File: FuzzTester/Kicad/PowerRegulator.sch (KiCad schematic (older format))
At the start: 18 parts, among them J5 TestPower_PinHeader, J6 9V Power JST XH, U1 AMS1117-5.0, U2 AMS1117-3.3, U22 LM2576HVS-ADJ

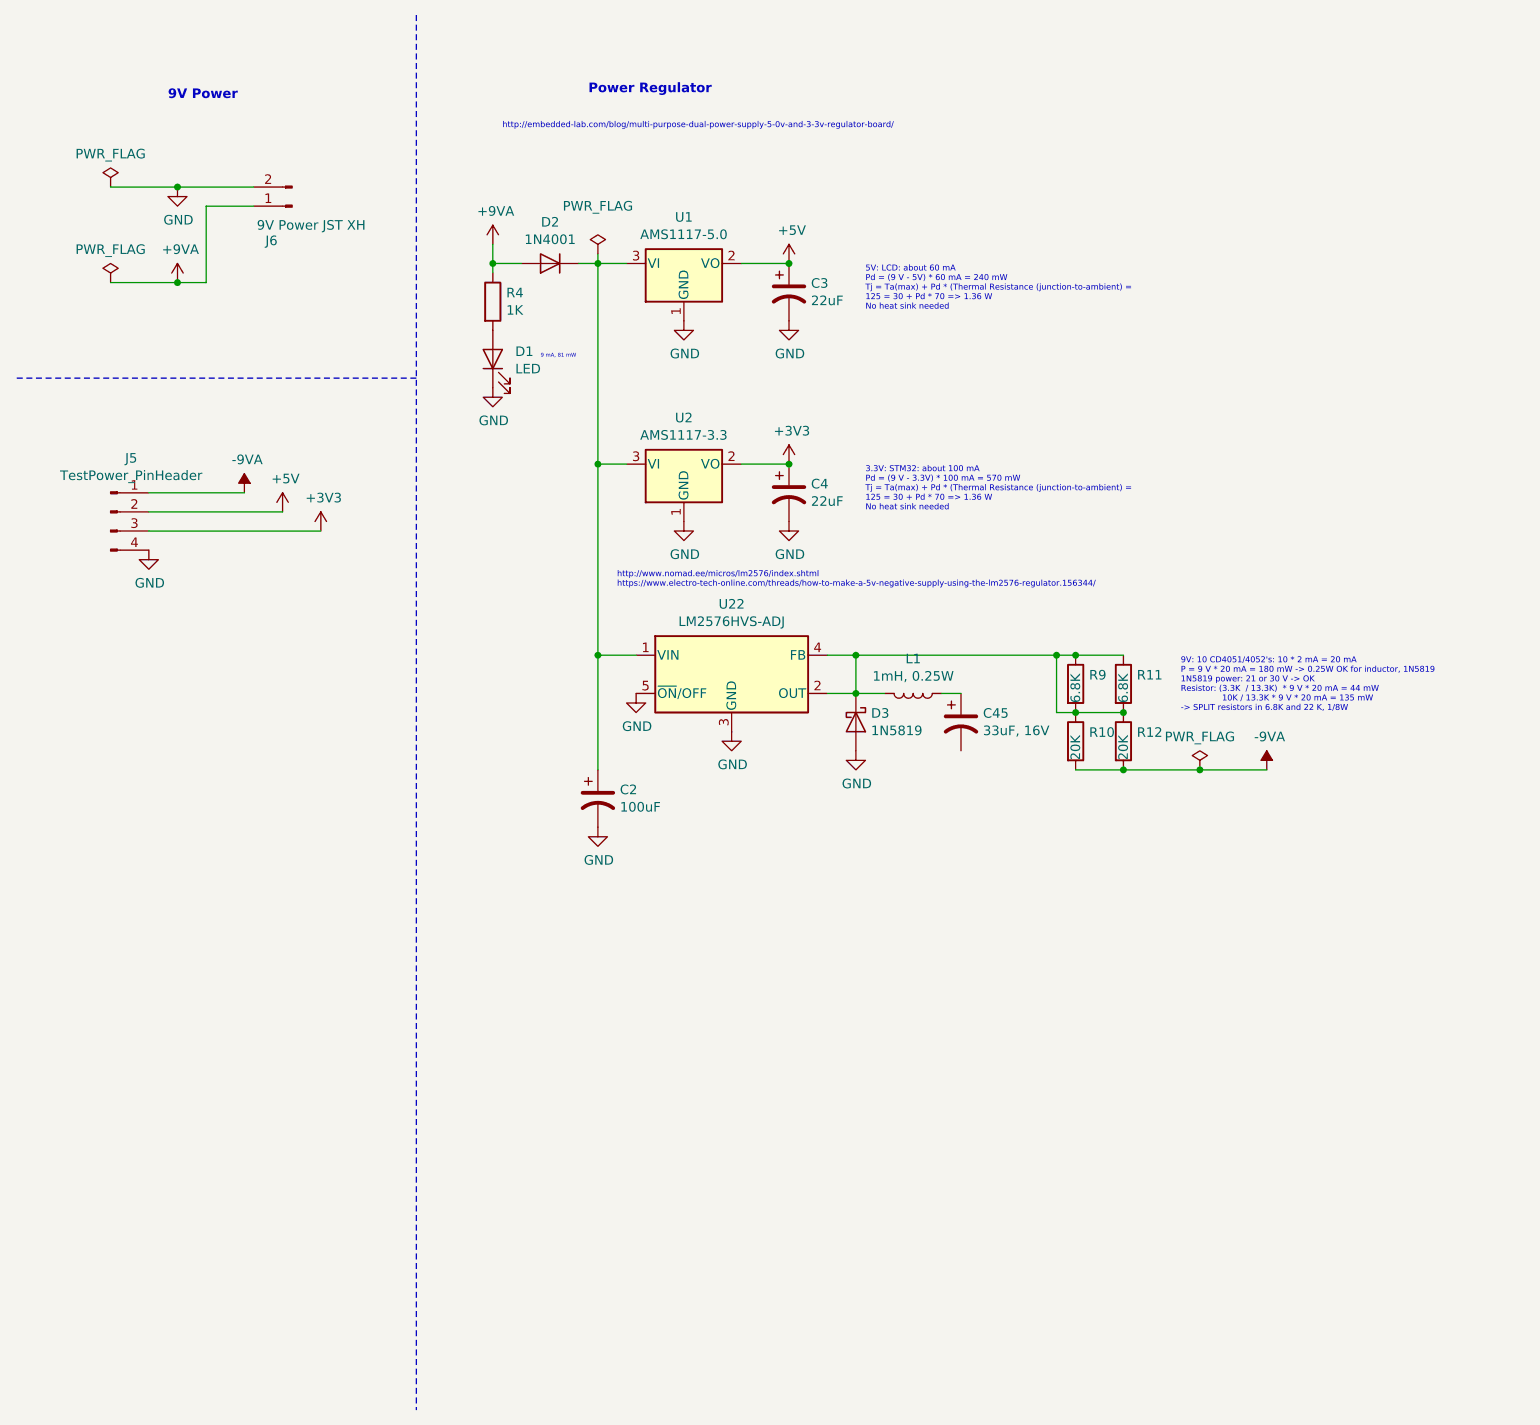
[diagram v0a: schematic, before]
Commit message: PCB Placement 100x82
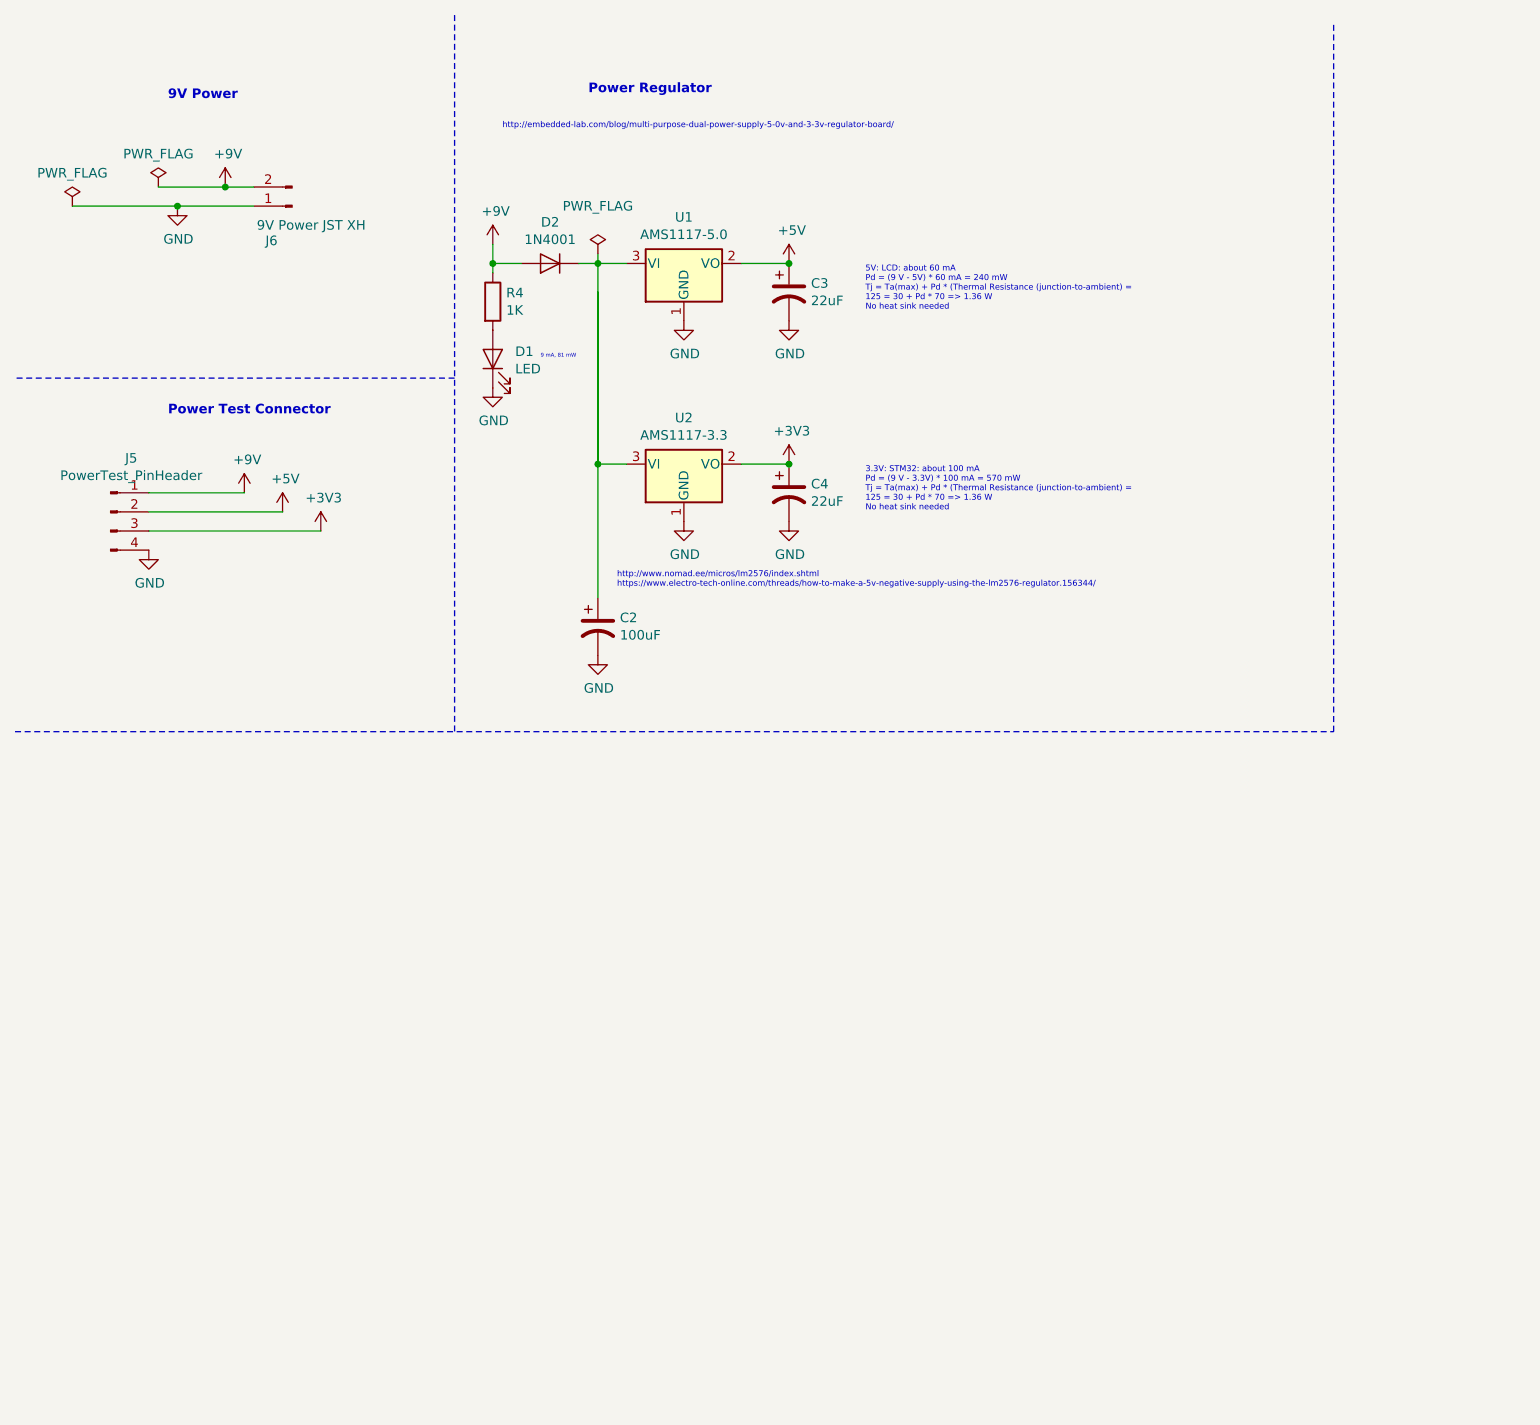
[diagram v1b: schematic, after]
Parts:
- removed C45: 33uF, 16V, symbol Device:CP1
- removed D3: 1N5819, Diode_THT:D_DO-41_SOD81_P10.16mm_Horizontal, symbol Diode:1N5819
- removed L1: 1mH, 0.25W, symbol Device:L
- removed R10, R12: 20K, symbol Device:R
- removed R11, R9: 6.8K, symbol Device:R
- removed U22: LM2576HVS-ADJ, Package_TO_SOT_SMD:TO-263-5_TabPin3, symbol Regulator_Switching:LM2576HVS-ADJ
- J5: value TestPower_PinHeader -> PowerTest_PinHeader; footprint (none) -> Connector_PinHeader_2.54mm:PinHeader_1x04_P2.54mm_Vertical
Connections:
- net labels added: +9V
- net labels removed: +9VA, -9VA
- wire segments 36 -> 19
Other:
- note added: "Power Test Connector\n"
- note removed: "9V: 10 CD4051/4052's: 10 * 2 mA = 20 mA\nP = 9 V * 20 mA = 180 mW -> 0.25W OK for inductor, 1N5819\n1N5819 power: 21 or 30 V -> OK\nResistor: (3.3K / 13.3K) * 9 V * 20 mA = 44 mW\n 10K / 13.3K * 9 V * 20 mA = 135 mW\n-> SPLIT resistors in 6.8K and 22 K, 1/8W\n"
- moved on the sheet: C2
